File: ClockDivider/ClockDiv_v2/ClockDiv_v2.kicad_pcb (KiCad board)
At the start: 2 copper layers, 50 x 127 mm, 39 parts, among them J1 Conn_02x05_Counter_Clockwise, J2 ClockIn, J3 ResetIn, J4 /2, J5 /4, J6 /8, J7 /16, J8 /32, J9 /64, Q1 2N3904, U1 4040, U2 L7805

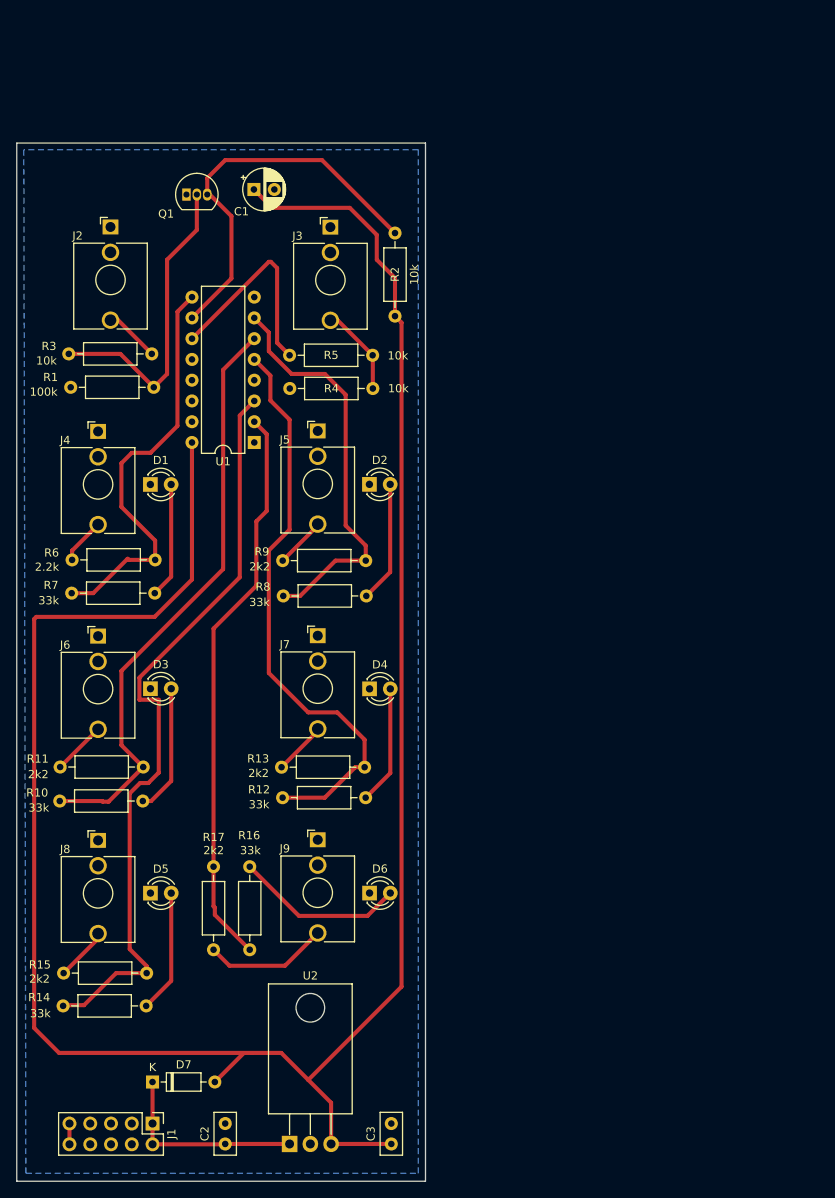
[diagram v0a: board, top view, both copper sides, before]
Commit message: Redesigned PCB
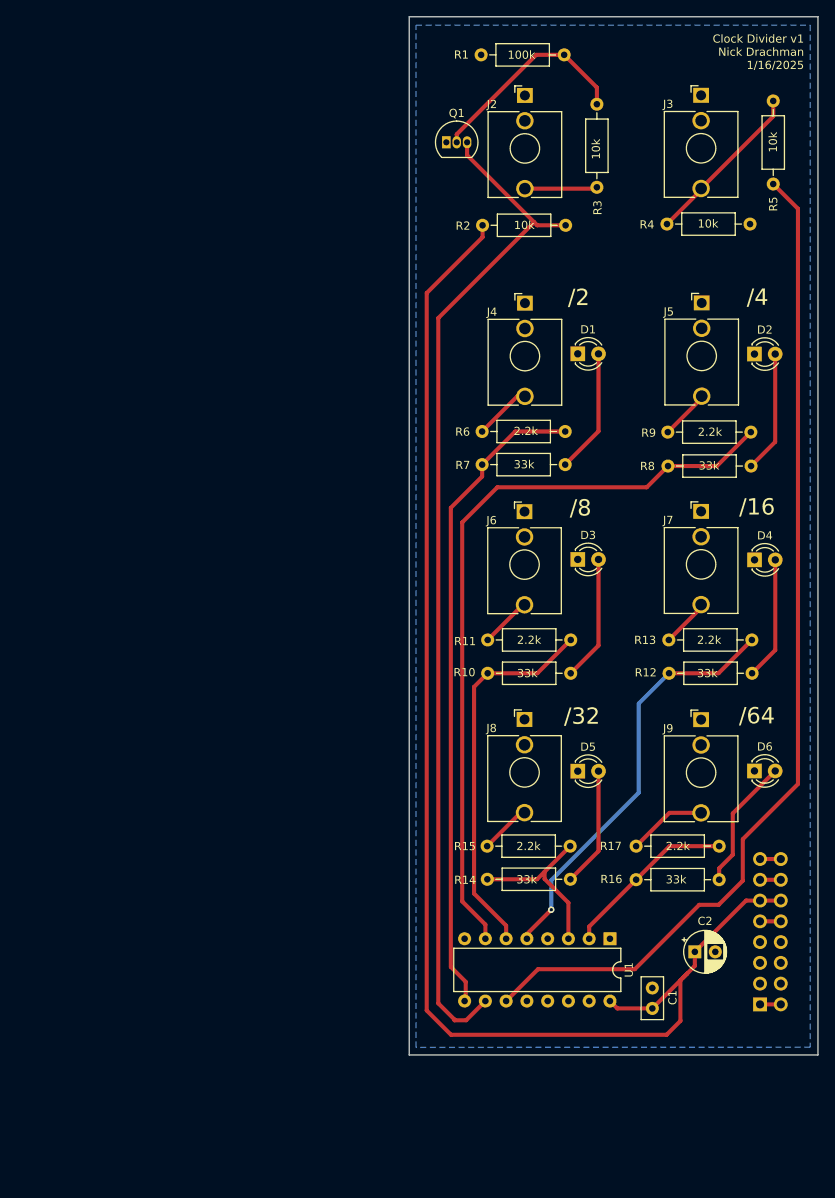
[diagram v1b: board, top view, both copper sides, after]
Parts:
- removed C3: 0.1u, Capacitor_THT:C_Disc_D5.0mm_W2.5mm_P2.50mm
- removed D7: 1N4148, Diode_THT:D_DO-35_SOD27_P7.62mm_Horizontal
- removed J1: Conn_02x05_Counter_Clockwise, Connector_PinHeader_2.54mm:PinHeader_2x05_P2.54mm_Vertical
- removed U2: L7805, Package_TO_SOT_THT:TO-220-3_Horizontal_TabDown
- added J10: Conn_02x08_Odd_Even, Connector_PinHeader_2.54mm:PinHeader_2x08_P2.54mm_Vertical, B.Cu at (158.1, 149.3)
- C1: footprint Capacitor_THT:CP_Radial_D5.0mm_P2.50mm -> Capacitor_THT:C_Disc_D5.0mm_W2.5mm_P2.50mm
- C2: value 0.33u -> 10u; footprint Capacitor_THT:C_Disc_D5.0mm_W2.5mm_P2.50mm -> Capacitor_THT:CP_Radial_D5.0mm_P2.50mm
- moved C1 111.4 mm to (145.0, 149.8), turned to 90 degrees
- moved U1 74.7 mm to (139.8, 141.2), turned to -90 degrees
- moved R3 71.5 mm to (138.2, 39.1), turned to -90 degrees
- moved R1 64.6 mm to (124.0, 33.1)
- moved R5 62.8 mm to (159.8, 48.9), turned to 90 degrees
- moved C2 62.1 mm to (150.2, 142.8), turned to 0 degrees
- moved D1 54.7 mm to (135.8, 69.7)
- moved R10 54.6 mm to (124.8, 108.8)
- moved D3 54.6 mm to (135.8, 94.8)
- moved R11 54.6 mm to (124.8, 104.7)
- moved J4 54.5 mm to (129.4, 63.5)
- moved D5 54.4 mm to (135.8, 120.7)
- moved J6 54.3 mm to (129.3, 89.0)
- moved J8 54.2 mm to (129.3, 114.4)
- moved R14 54.2 mm to (124.8, 133.9)
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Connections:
- C1 pad 1: Net-(D7-A) -> +5V
- C2 pad 1: +12V -> +5V
- R2 pad 1: Net-(D7-A) -> +5V
- U1 pad 16: Net-(D7-A) -> +5V
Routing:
- net Net-(D7-A): track 273.4 -> 0.00 mm
- net +5V: track 0.00 -> 165.4 mm
- net Net-(U1-Reset): track 25.9 -> 124.3 mm
- net Net-(Q1-C): track 48.1 -> 125.2 mm
- net Net-(U1-Q4): track 93.0 -> 21.2 mm
- net Net-(U1-Q5): track 69.8 -> 21.5 mm
- net Net-(U1-Q1): track 49.6 -> 92.0 mm
- net Net-(U1-Q0): track 50.8 -> 79.9 mm
- net Net-(U1-Q2): track 72.2 -> 46.6 mm
- net +12V: track 24.4 -> 2.54 mm
- net Net-(U1-Q3): track 71.2 -> 51.5 mm, vias 0 -> 1
- net Net-(Q1-B): track 37.9 -> 25.8 mm
- net Net-(J3-PadT): track 11.0 -> 20.4 mm
- net Net-(J9-PadT): track 15.2 -> 9.64 mm
- net Net-(D6-A): track 20.8 -> 16.1 mm
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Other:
- board text added: "/16"
- board text added: "/2"
- board text added: "/32"
- board text added: "/4"
- board text added: "/64"
- board text added: "/8"
- board text added: "100k"
- board text added: "10k"
- board text added: "2.2k"
- board text added: "33k"
- board text added: "Clock Divider v1 Nick Drachman 1/16/2025"
